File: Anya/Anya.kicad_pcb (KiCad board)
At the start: 2 copper layers, 190.5 x 76.2 mm, 77 parts, among them SW1 SW_Push, SW10 SW_Push, SW11 SW_Push, SW12 SW_Push, SW13 SW_Push, SW14 SW_Push, SW15 SW_Push, SW16 SW_Push, SW17 SW_Push, SW18 SW_Push, SW19 SW_Push, SW2 SW_Push, SW20 SW_Push, SW21 SW_Push, SW22 SW_Push, SW23 SW_Push, SW24 SW_Push, SW25 SW_Push, SW26 SW_Push, SW27 SW_Push, SW28 SW_Push, SW29 SW_Push, SW3 SW_Push, SW30 SW_Push, SW31 SW_Push, SW32 SW_Push, SW33 SW_Push, SW4 SW_Push, SW5 SW_Push, SW6 SW_Push, SW7 SW_Push, SW8 SW_Push, SW9 SW_Push, U1 ProMicro

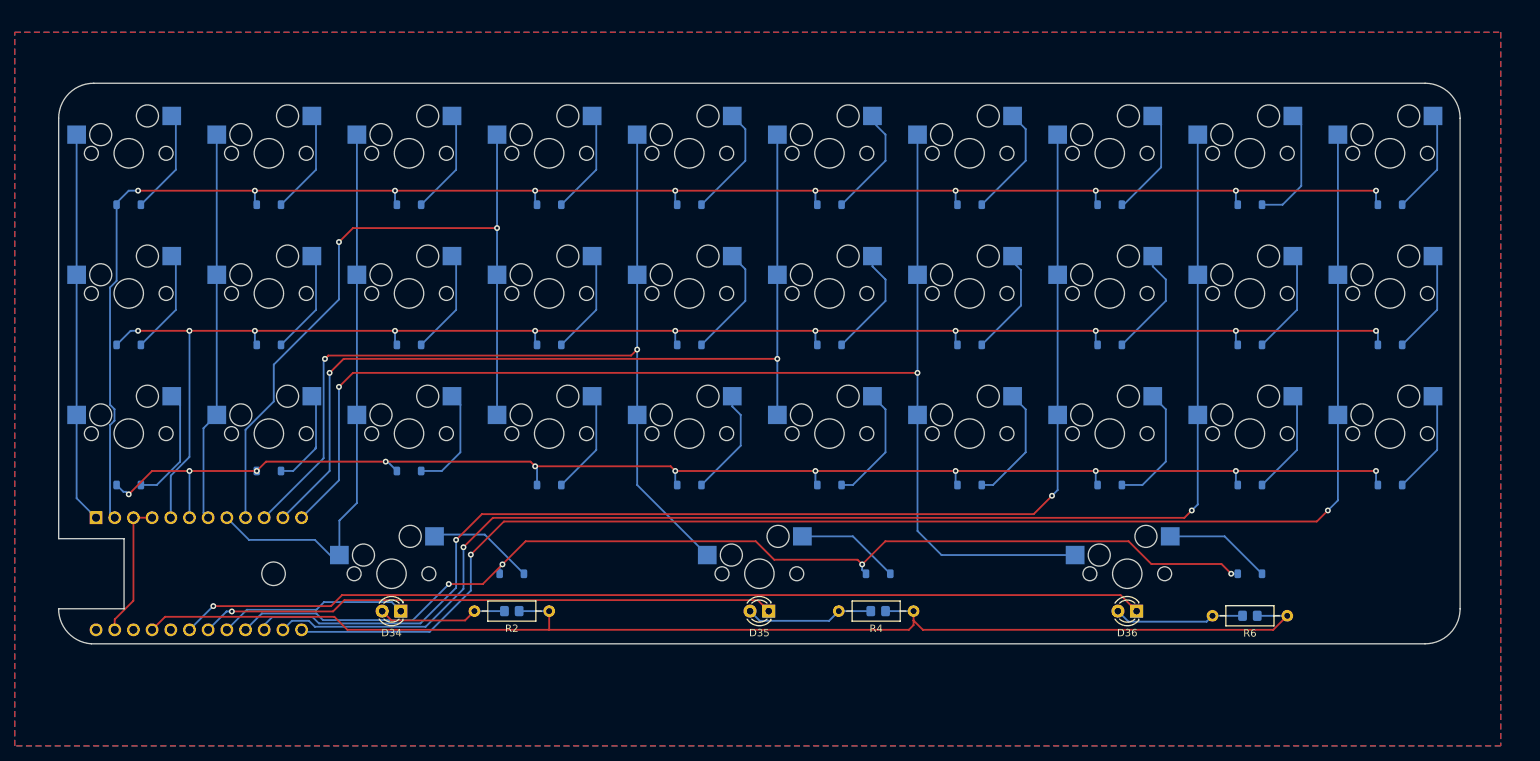
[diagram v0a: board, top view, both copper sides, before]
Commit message: anya r2
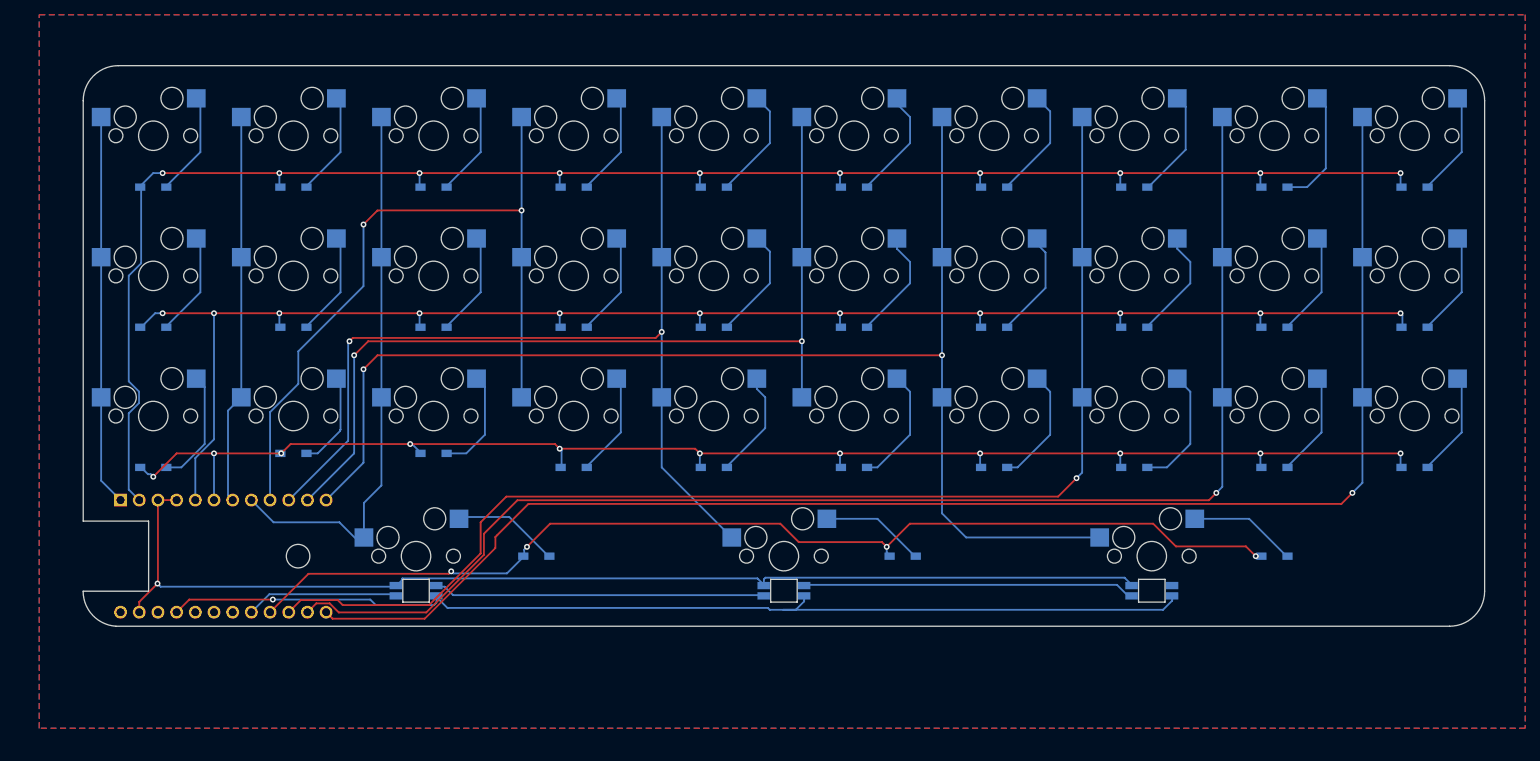
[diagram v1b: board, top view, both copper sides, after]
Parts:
- removed D34, D35, D36: LED, LED_THT:LED_D3.0mm
- removed R1, R3, R5: R, Resistor_SMD:R_0805_2012Metric_Pad1.20x1.40mm_HandSolder
- removed R2, R4, R6: R, Resistor_THT:R_Axial_DIN0207_L6.3mm_D2.5mm_P10.16mm_Horizontal
- added LED1: YS-SK6812MINI-E, Keyboard_JSA:YS-SK6812MINI-E, B.Cu at (102.6, 103.9)
- added LED2: YS-SK6812MINI-E, Keyboard_JSA:YS-SK6812MINI-E, B.Cu at (152.6, 103.9)
- added LED3: YS-SK6812MINI-E, Keyboard_JSA:YS-SK6812MINI-E, B.Cu at (202.6, 103.9)
- D1, D10, D11, D12, D13, D14, D15, D16, D17, D18, D19, D2, D20, D21, D22, D23, D24, D25, D26, D27, D28, D29, D3, D30, D31, D32, D33, D4, D5, D6, D7, D8, D9: footprint Diode_SMD:D_SOD-123 -> Keyboard_JSA:D3_SMD_v2
- moved D10 4.10 mm to (238.3, 49.0)
- moved D12 4.10 mm to (85.9, 68.1)
- moved D13 4.10 mm to (104.9, 68.1)
- moved D15 4.10 mm to (143.0, 68.1)
- moved D16 4.10 mm to (162.1, 68.1)
- moved D18 4.10 mm to (200.2, 68.1)
- moved D19 4.10 mm to (219.2, 68.1)
- moved D2 4.10 mm to (85.9, 49.0)
- moved D20 4.10 mm to (238.3, 68.1)
- moved D22 4.10 mm to (85.9, 85.2)
- moved D23 4.10 mm to (104.9, 85.2)
- moved D25 4.10 mm to (143.0, 87.1)
- moved D26 4.10 mm to (162.1, 87.1)
- moved D28 4.10 mm to (200.2, 87.1)
- moved D29 4.10 mm to (219.2, 87.1)
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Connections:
- U1 pad 17: Left -> Net-(LED1-DIN)
- U1 pad 18: Middle -> unconnected-(U1-A1/PF6-Pad18)
- U1 pad 19: Right -> unconnected-(U1-A2/PF5-Pad19)
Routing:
- net GND: track 18.8 -> 153.7 mm, vias 0 -> 1
- net Right: track 131.6 -> 0.00 mm, vias 1 -> 0
- net Middle: track 78.5 -> 0.00 mm, vias 1 -> 0
- net Net-(LED2-DOUT): track 0.00 -> 45.1 mm
- net Net-(LED1-DOUT): track 0.00 -> 45.0 mm
- net VCC: track 173.8 -> 143.3 mm, vias 0 -> 1
- net Left: track 25.7 -> 0.00 mm
- net Net-(LED1-DIN): track 0.00 -> 20.8 mm
- net Net-(D36-A): track 17.9 -> 0.00 mm
- net Net-(D34-A): track 17.7 -> 0.00 mm
- net Net-(D35-A): track 17.5 -> 0.00 mm
- net Row 4: track 148.0 -> 146.5 mm
- net Row 1: track 231.4 -> 232.7 mm
- net Col 9: track 185.7 -> 184.4 mm, vias 2 -> 1
- net Col 8: track 168.3 -> 167.1 mm, vias 2 -> 1
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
